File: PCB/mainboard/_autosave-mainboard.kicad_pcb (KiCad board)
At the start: 2 copper layers, 100 x 68 mm, 1 part, among them IC1 STM32H743ZIT6

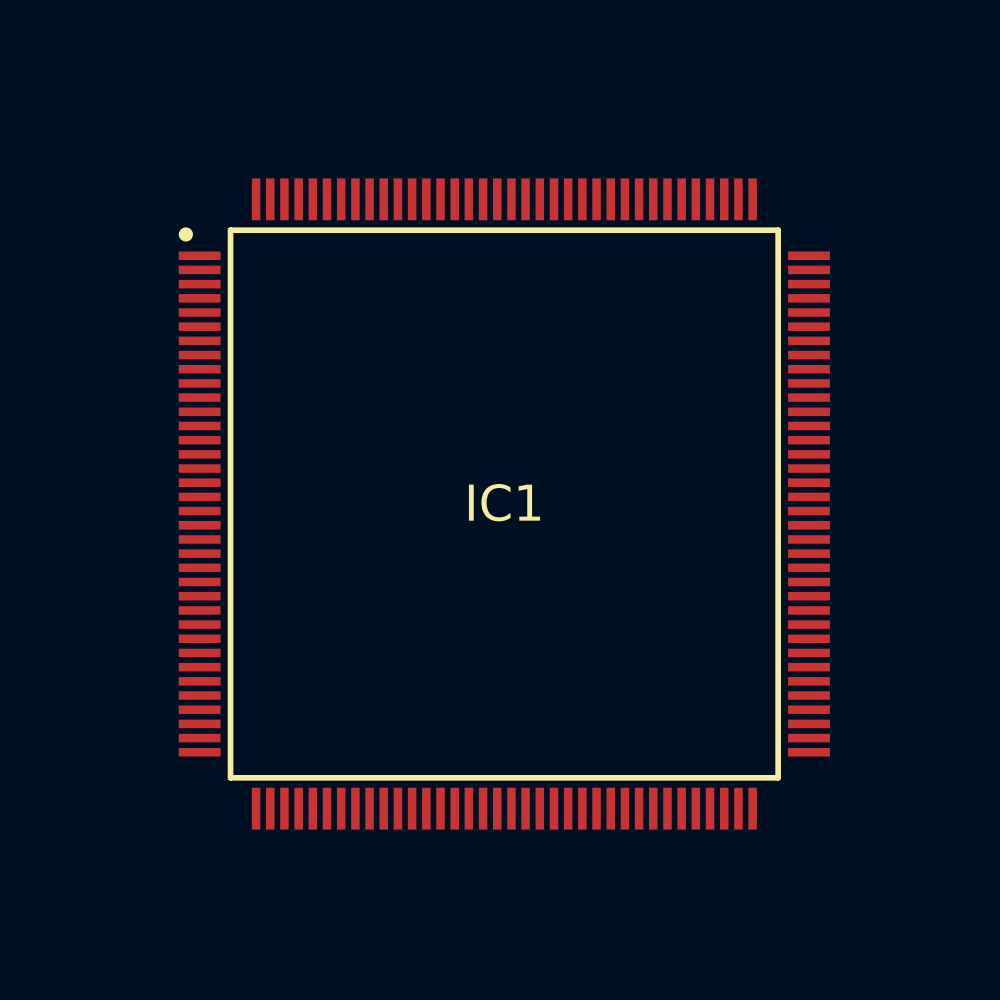
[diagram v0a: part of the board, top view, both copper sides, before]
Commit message: STM32 Mainboard requirements for Programing and Power
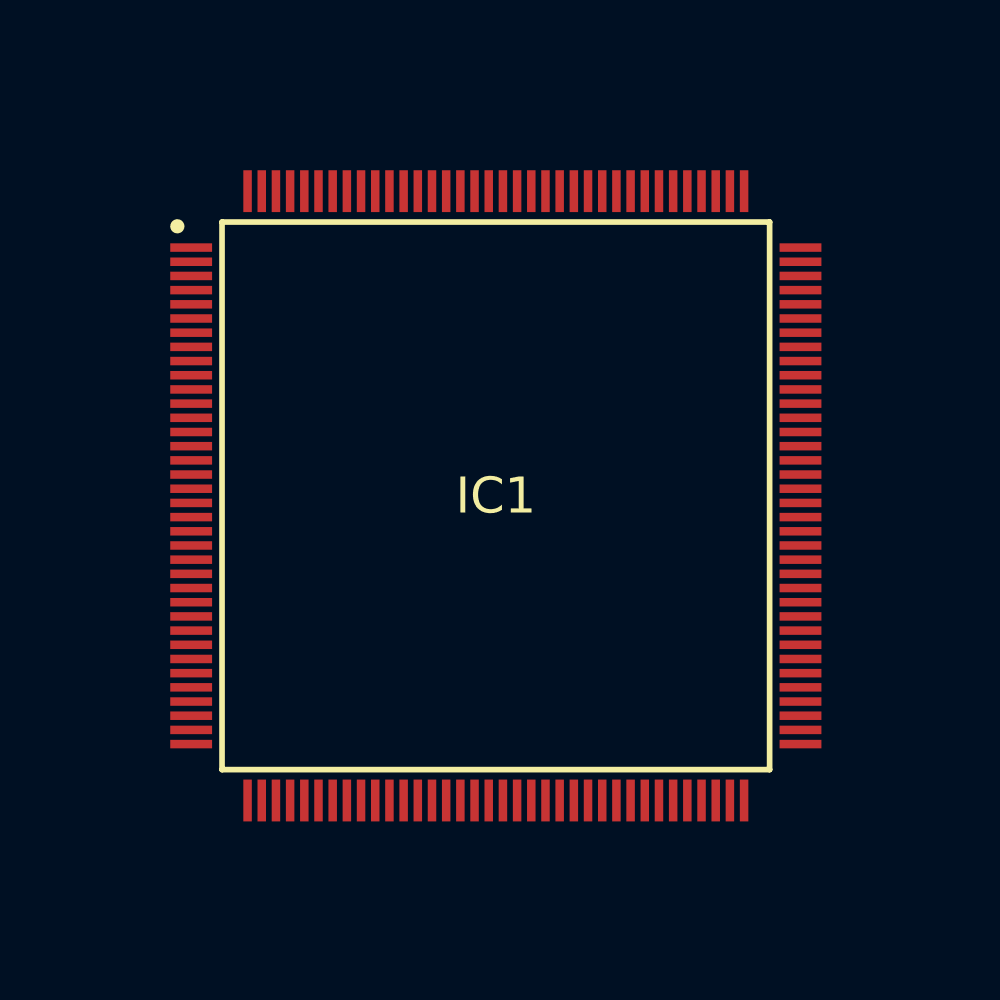
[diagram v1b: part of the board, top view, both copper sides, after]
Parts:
- moved IC1 0.42 mm to (149.2, 103.8)
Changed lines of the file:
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@@
 	(footprint "lib:QFP50P2200X2200X160-144N"
 		(layer "F.Cu")
-		(at 149.55 104.038)
+		(at 149.25 103.75)
 		(descr "LQFP144, 20 x 20 mm, 144-pin")
 		(tags "Integrated Circuit")
